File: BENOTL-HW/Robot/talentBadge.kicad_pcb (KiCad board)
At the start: 2 copper layers, 93.8 x 102.7 mm, 65 parts, among them P1 USB_A, P2 OLED, P3 Batt, P4 PS, P5 sd_card_spi, Q1 MMBT3904, Q2 MMBT3904, Q3 IR phototransistor, SW1 B1, SW2 B2, SW3 RST, U1 esp8266-12, U10 ws2812b, U11 ws2812b, U12 ws2812b, U13 ws2812b, U14 ws2812b, U15 ws2812b, U16 ws2812b, U2 CP2102N, U3 SP0503BAHTG, U4 AP111733, U5 ws2812b, U6 ws2812b, U7 ws2812b, U8 ws2812b, U9 ws2812b

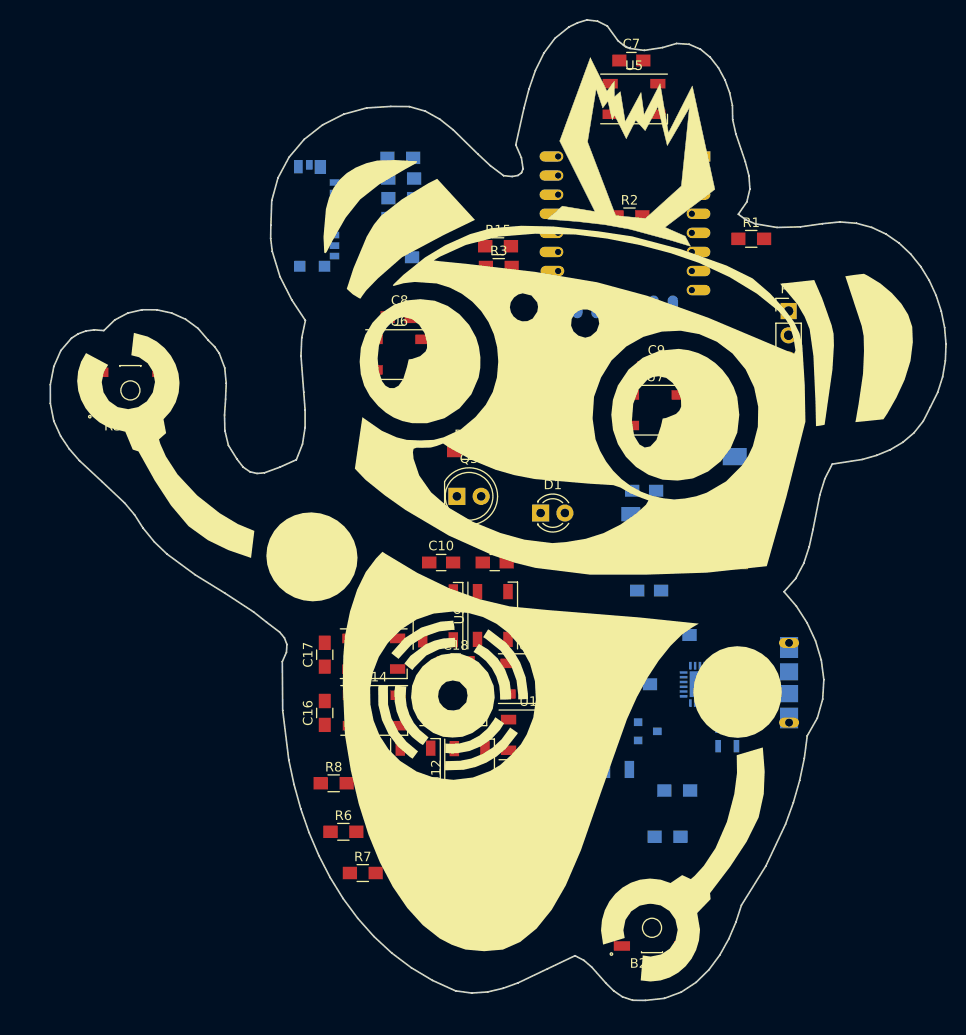
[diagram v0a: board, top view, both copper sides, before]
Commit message: Routeo para revision
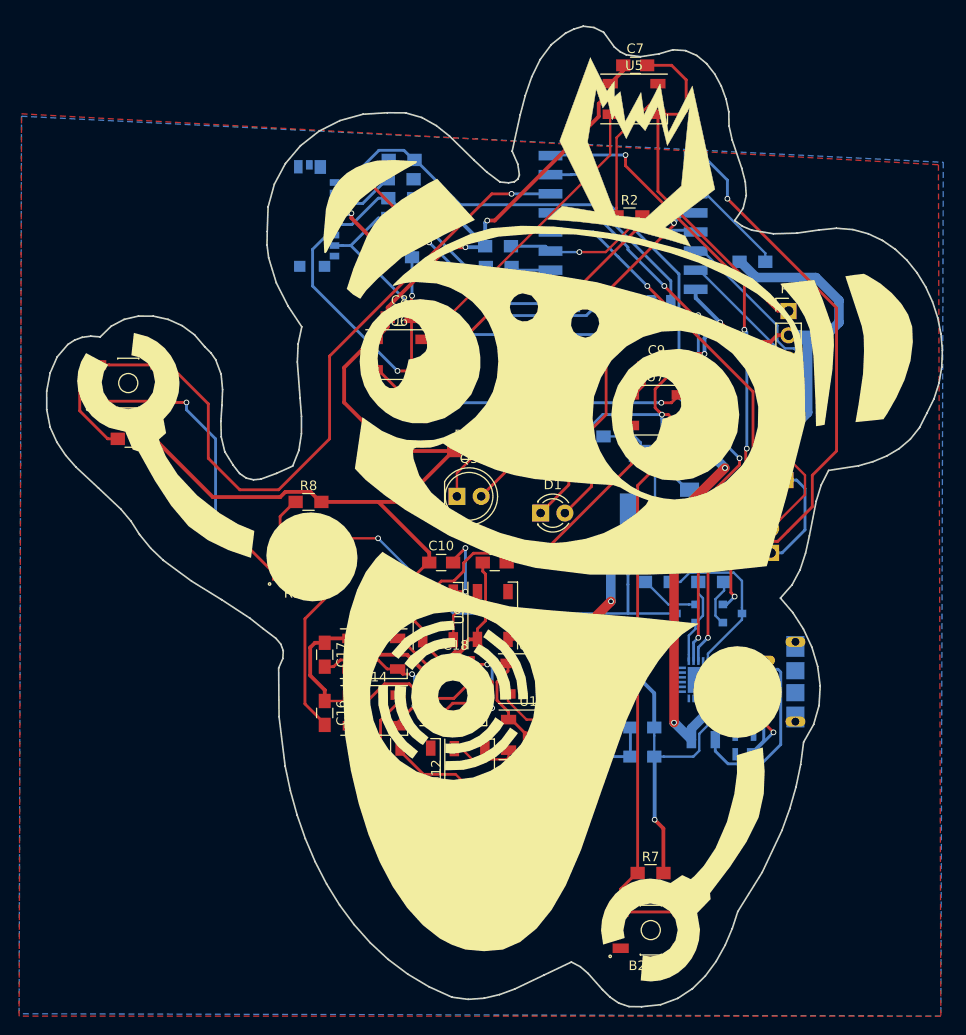
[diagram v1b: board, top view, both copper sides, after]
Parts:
- R1, R15, R3: moved to B.Cu
- U1: footprint ESP8266:ESP-12E -> RF_Modules:ESP-12E
- moved SW1 64.4 mm to (36.6, 91.4)
- moved R6 46.8 mm to (36.8, 97.3)
- moved R7 30.1 mm to (91.3, 142.7)
- moved R8 29.6 mm to (55.5, 103.9)
- moved R4 26.7 mm to (92.0, 112.3)
- moved SW3 25.7 mm to (55.6, 109.7)
- moved R5 22.1 mm to (97.6, 112.3), turned to 180 degrees
- moved Q2 15.2 mm to (99.8, 115.6)
- moved C1 13.3 mm to (90.4, 130.6), turned to 180 degrees
- moved F1 11.9 mm to (98.0, 128.8), turned to 180 degrees
- moved Q1 8.59 mm to (95.0, 115.6), turned to 180 degrees
- moved U1 7.96 mm to (88.4, 71.1)
- moved C3 7.92 mm to (85.1, 97.0), turned to 180 degrees
- moved C4 5.91 mm to (85.9, 110.5), turned to 180 degrees
- moved D2 5.86 mm to (92.2, 98.8)
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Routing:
- net +3V3: track 0.00 -> 387.3 mm, vias 0 -> 11
- net GND: track 0.00 -> 274.7 mm, vias 0 -> 17
- net RST: track 0.00 -> 120.2 mm, vias 0 -> 3
- net B2: track 0.00 -> 93.8 mm, vias 0 -> 3
- net B1: track 0.00 -> 84.8 mm, vias 0 -> 1
- net TXD: track 0.00 -> 68.2 mm, vias 0 -> 4
- net RXD: track 0.00 -> 62.9 mm, vias 0 -> 2
- net GPIO0: track 0.00 -> 52.3 mm, vias 0 -> 2
- net CS: track 0.00 -> 45.5 mm
- net MISO: track 0.00 -> 44.2 mm
- net IRT: track 0.00 -> 44.0 mm, vias 0 -> 1
- net /VBUS: track 0.00 -> 42.1 mm, vias 0 -> 2
- net MOSI: track 0.00 -> 38.8 mm, vias 0 -> 2
- net IRL: track 0.00 -> 37.8 mm, vias 0 -> 1
- net Net-(C3-Pad1): track 0.00 -> 34.9 mm, vias 0 -> 1
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- added copper zone on B.Cu, net GND
- added copper zone on F.Cu, net GND
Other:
- net class Default: trace_width 0.25 -> 0.3
- net class VCC added: clearance 0.2, trace_width 0.4, via_dia 0.6, via_drill 0.4
